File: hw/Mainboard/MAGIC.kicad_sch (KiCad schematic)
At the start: 15 parts, among them U18 SN74LVC4245APWR, U19 SN74LVC4245APWR, U20 SN74LVC4245APWR

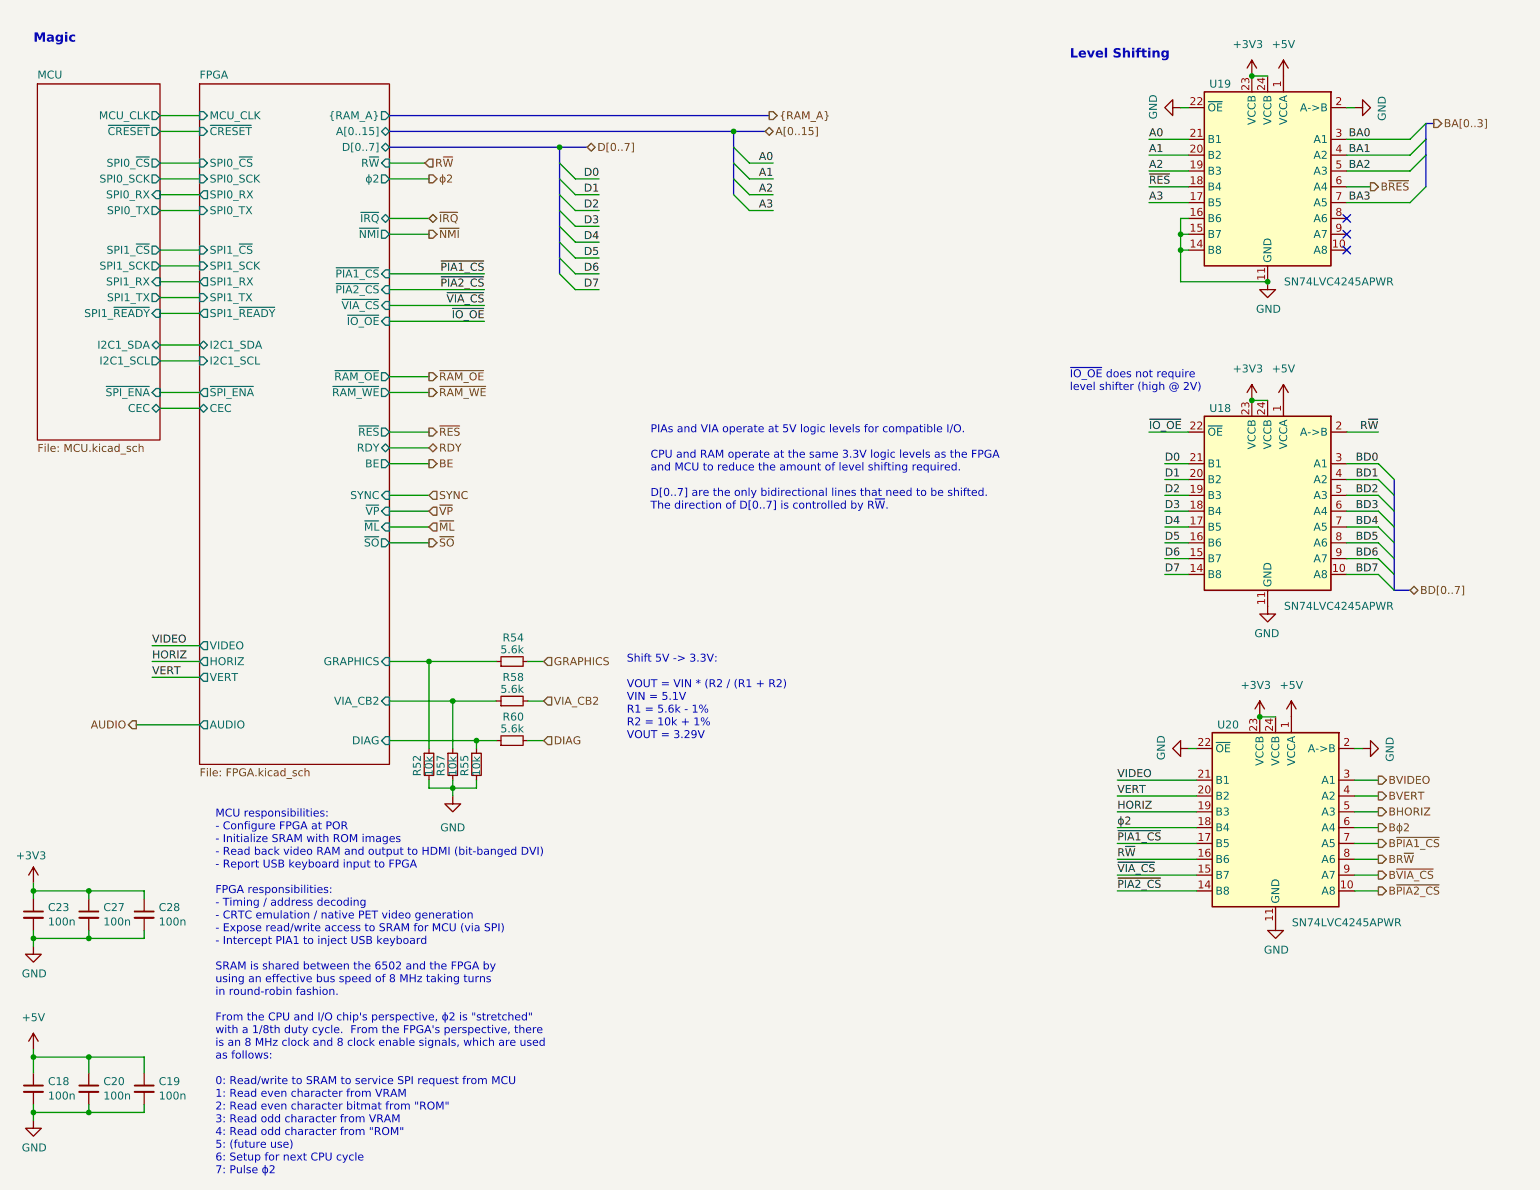
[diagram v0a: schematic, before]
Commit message: hw: wip
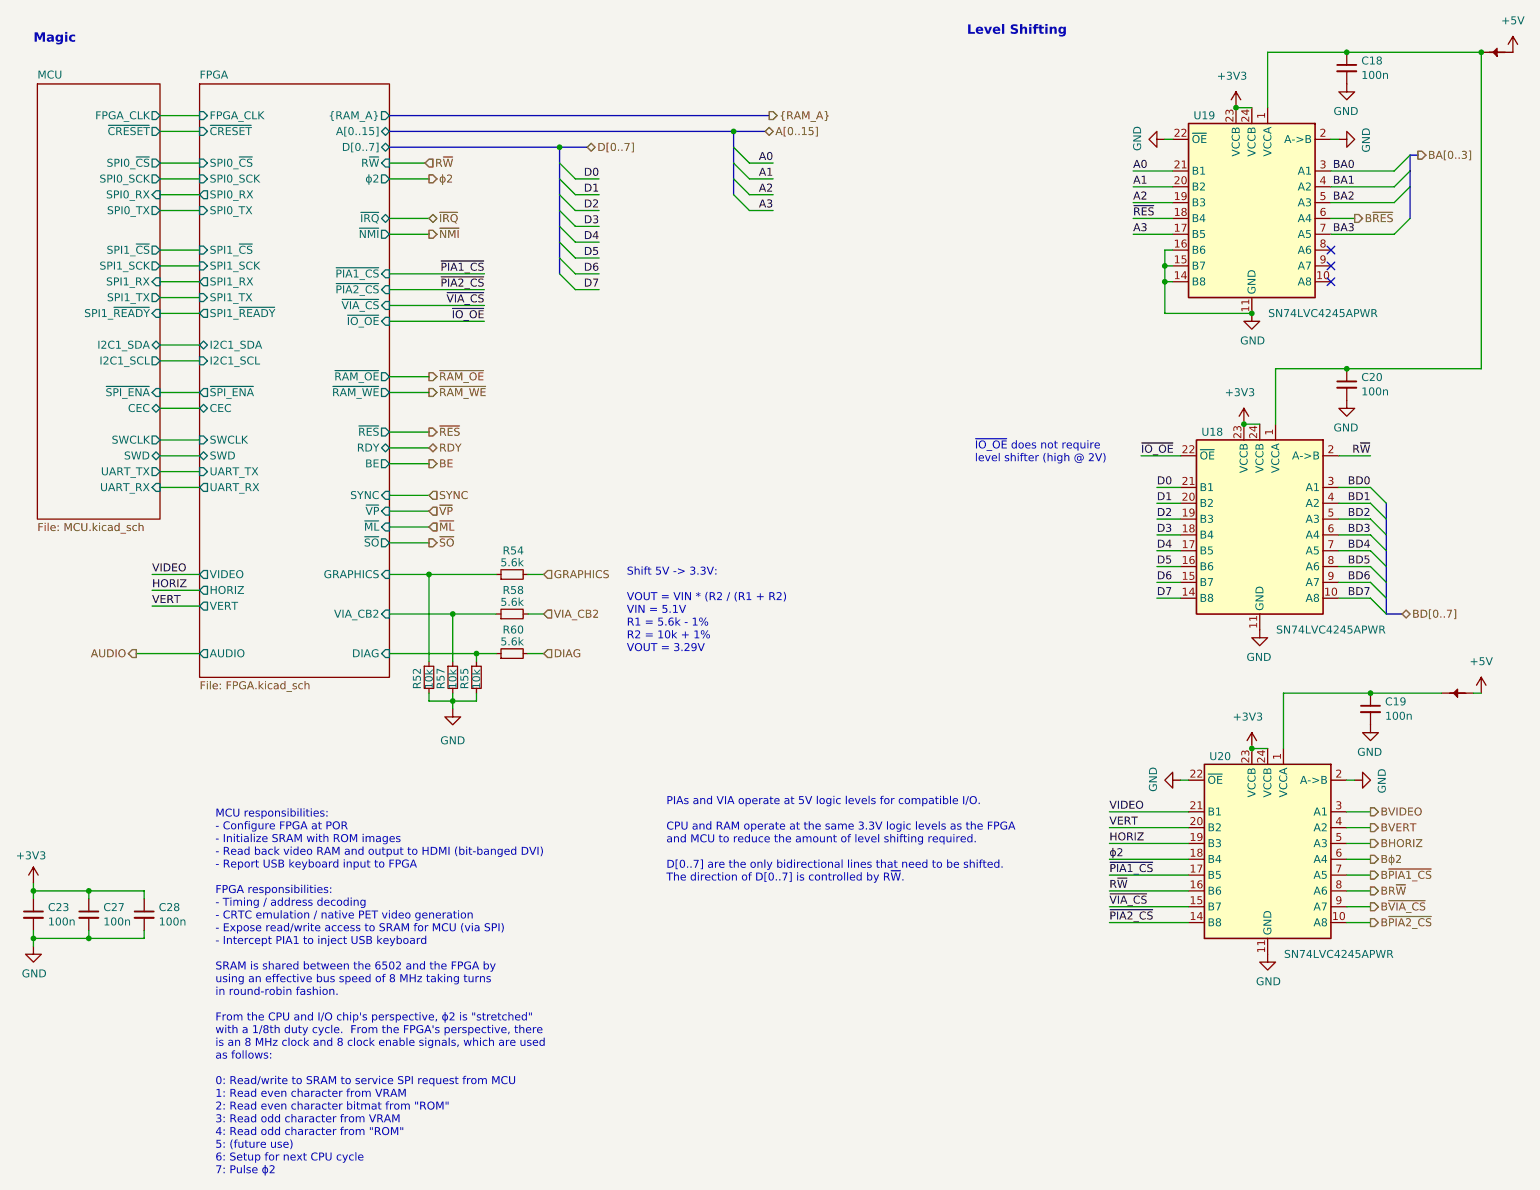
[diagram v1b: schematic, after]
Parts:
- added PT12, PT13: PowerTie_2, PET:NetTie-2_SMD_Pad_1.6_to_0.4mm, symbol PET:PowerTie_2
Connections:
- net +5V: now also PT12.1, PT13.1; no longer C18.1, C19.1, C20.1, U18.1 (VCCA), U19.1 (VCCA), U20.1 (VCCA)
- new net: C18.1, C20.1, PT12.2, U18.1 (VCCA), U19.1 (VCCA)
- new net: C19.1, PT13.2, U20.1 (VCCA)
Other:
- sheet FPGA ports: added FPGA_CLK, SWCLK, SWD, UART_RX, UART_TX; removed MCU_CLK
- sheet MCU ports: added FPGA_CLK, SWCLK, SWD, UART_RX, UART_TX; removed MCU_CLK
- moved on the sheet: C18, C19, C20, R52, R54, R55, R57, R58, R60, U18, U19, U20

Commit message: wip: support 8x16 keyboard matrix
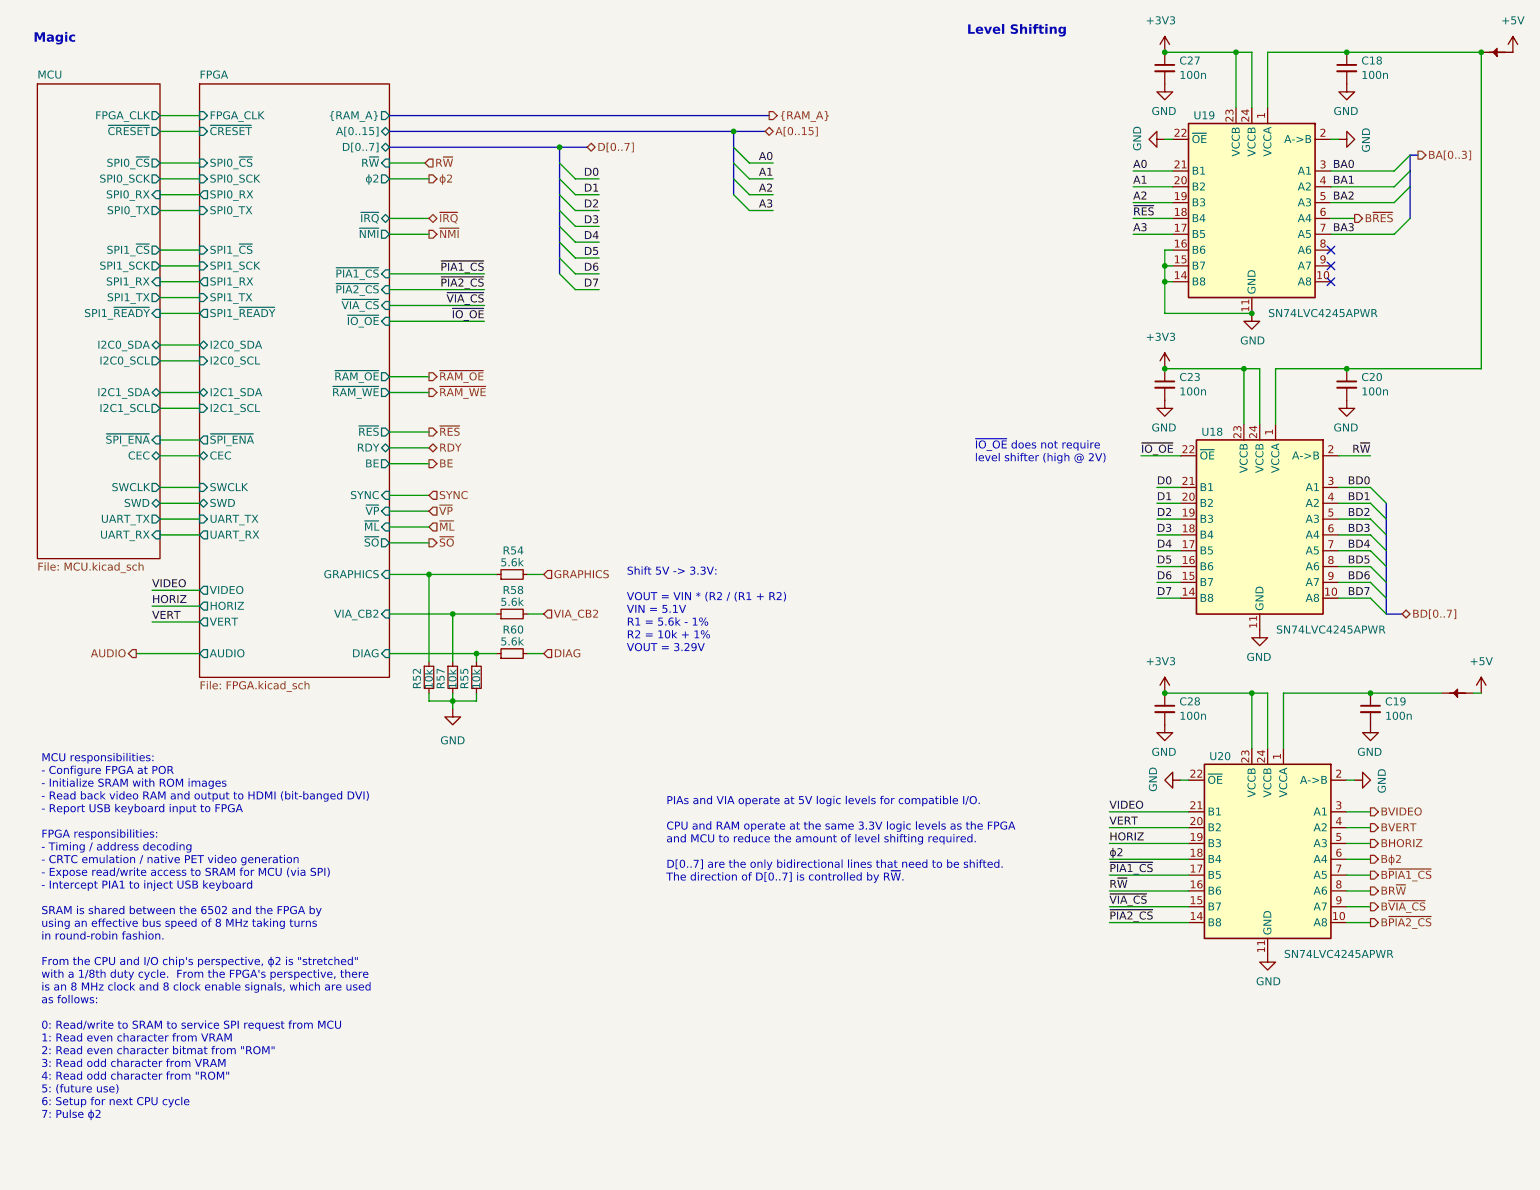
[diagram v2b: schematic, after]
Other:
- sheet FPGA ports: added I2C0_SCL, I2C0_SDA; removed none
- sheet MCU ports: added I2C0_SCL, I2C0_SDA; removed none
- moved on the sheet: C23, C27, C28
